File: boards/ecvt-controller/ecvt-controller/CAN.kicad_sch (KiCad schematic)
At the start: 23 parts, among them SW1 SW_SPST, SW2 SW_SPST, U1 TJA1051T-3, U3 MCP2515-xSO, U5 ACT45B-101-2P-TL003, U6 PESD2CAN,215, Y2 ABM3-16.000MHZ-D2Y-T

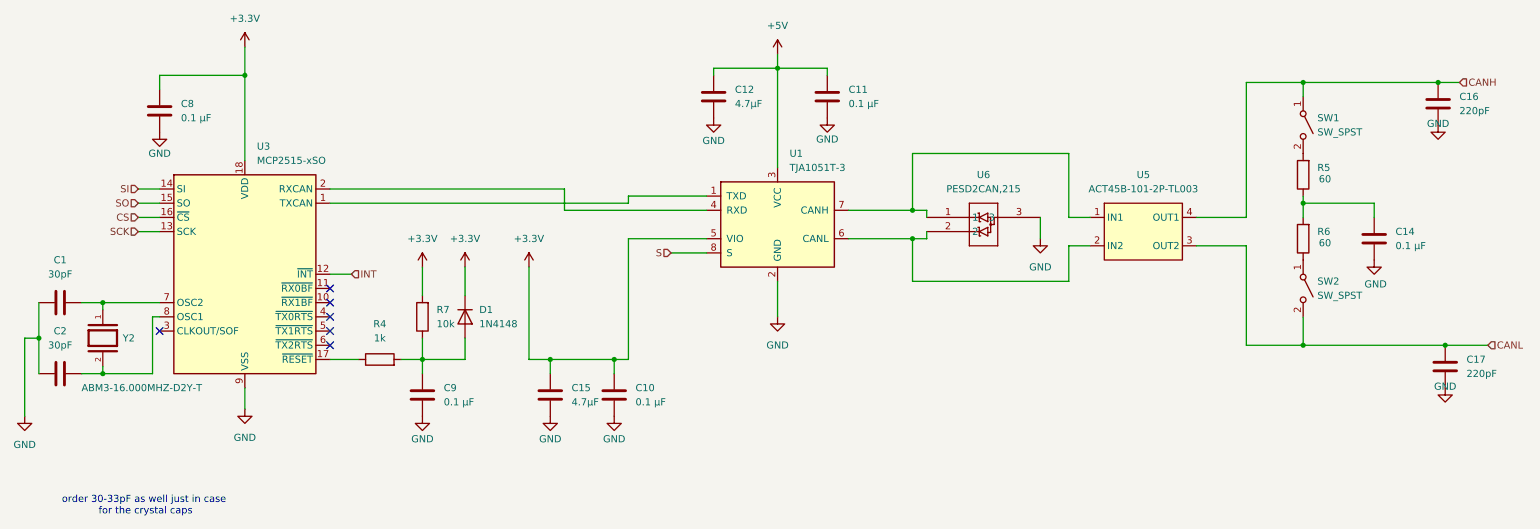
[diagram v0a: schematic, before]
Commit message: Resistors
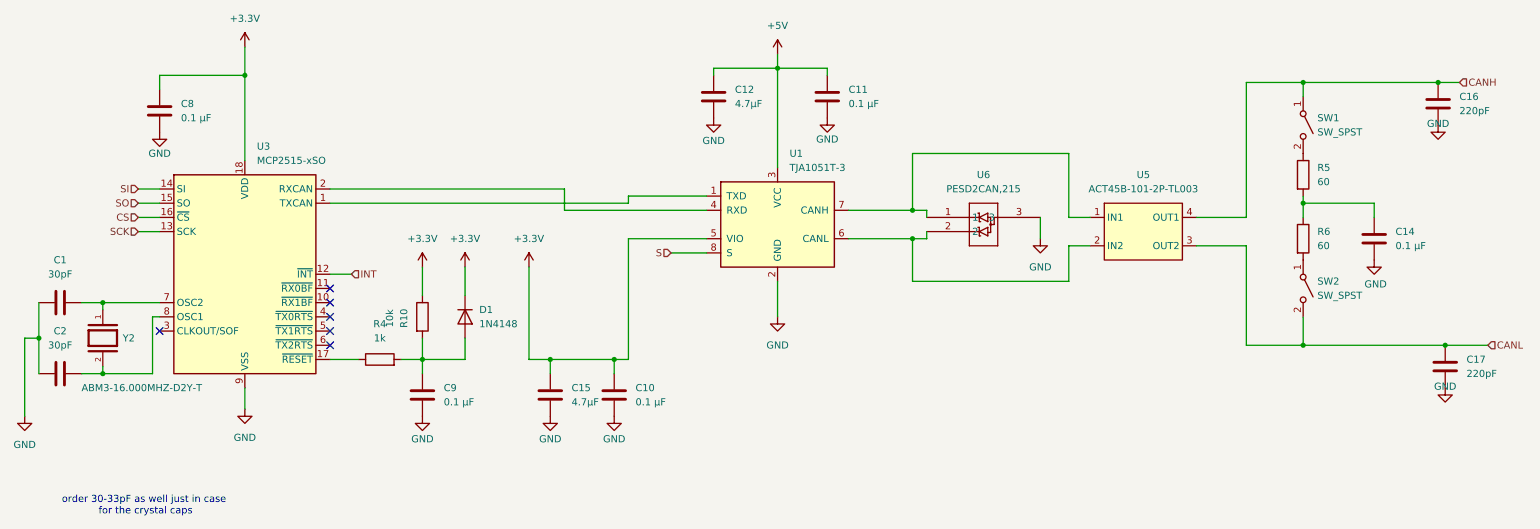
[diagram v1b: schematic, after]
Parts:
- removed R4: 1k, Resistor_SMD:R_0603_1608Metric_Pad0.98x0.95mm_HandSolder, symbol Device:R
- removed R5, R6: 60, Resistor_SMD:R_1206_3216Metric_Pad1.30x1.75mm_HandSolder, symbol Device:R
- removed R7: 10k, Resistor_SMD:R_0603_1608Metric_Pad0.98x0.95mm_HandSolder, symbol Device:R
- added R10: 10k, Resistor_SMD:R_0603_1608Metric_Pad0.98x0.95mm_HandSolder, symbol baja-common-parts:R_0603
- added R4: 1k, Resistor_SMD:R_0805_2012Metric_Pad1.20x1.40mm_HandSolder, symbol baja-common-parts:R_0805
- added R5, R6: 60, Resistor_SMD:R_0603_1608Metric_Pad0.98x0.95mm_HandSolder, symbol baja-common-parts:R_0603
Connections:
- net +3.3V: now also R10.1
- net at SW2.1 (A): now also R6.2
- net at C9.1, D1.2 (A): now also R10.2, R4.2
- net at U3.17 (~{RESET}): now also R4.1
- net at C14.1: now also R5.2, R6.1
- net at SW1.2 (B): now also R5.1
